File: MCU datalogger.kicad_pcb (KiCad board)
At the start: 2 copper layers, 50.8 x 30.5 mm, 29 parts, among them J1 Conn_01x04_Pin, J2 Conn_01x04_Pin, J3 Conn_01x09_Pin, J4 Conn_02x03_Odd_Even, U1 24LC1025, U2 24LC1025, U3 DS1337S_, U4 ATMEGA328P-AU, Y1 32.768 KHz, Y2 16 MHz

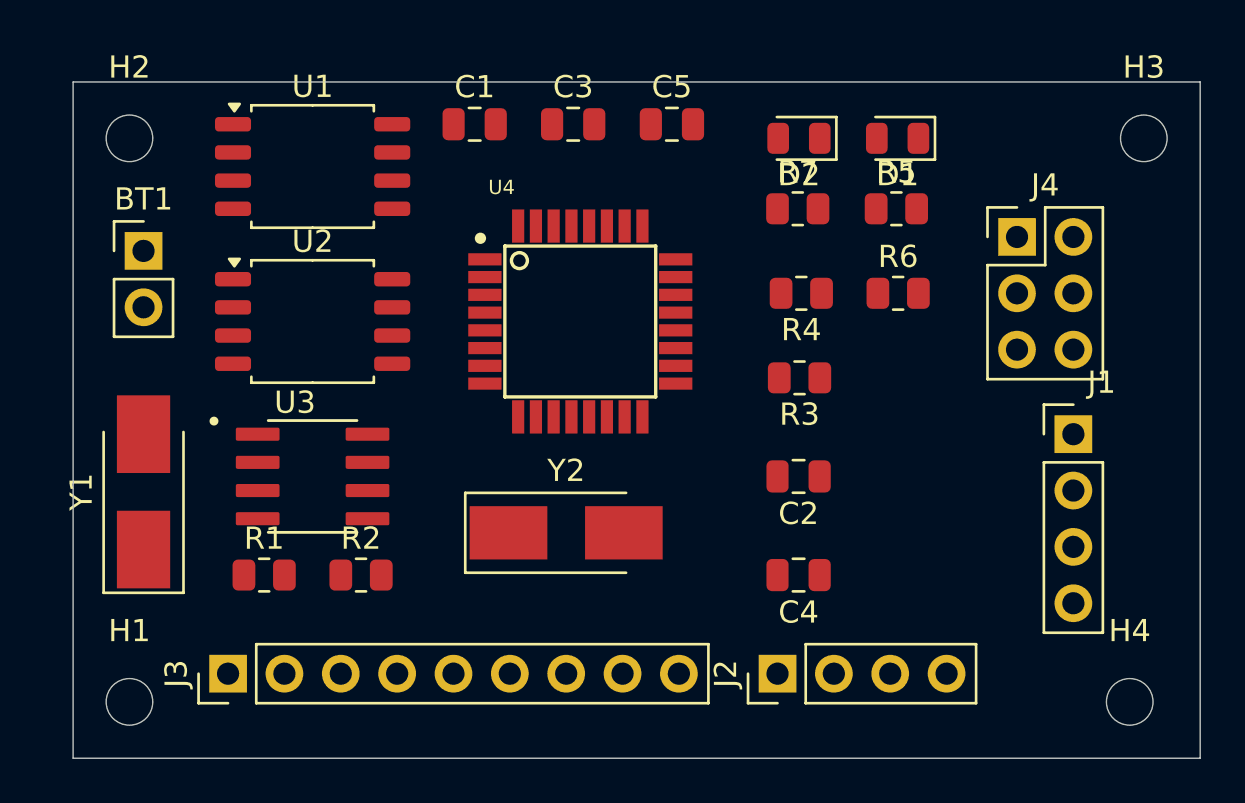
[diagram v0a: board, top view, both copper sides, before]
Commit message: Routing and GND Vcc complete
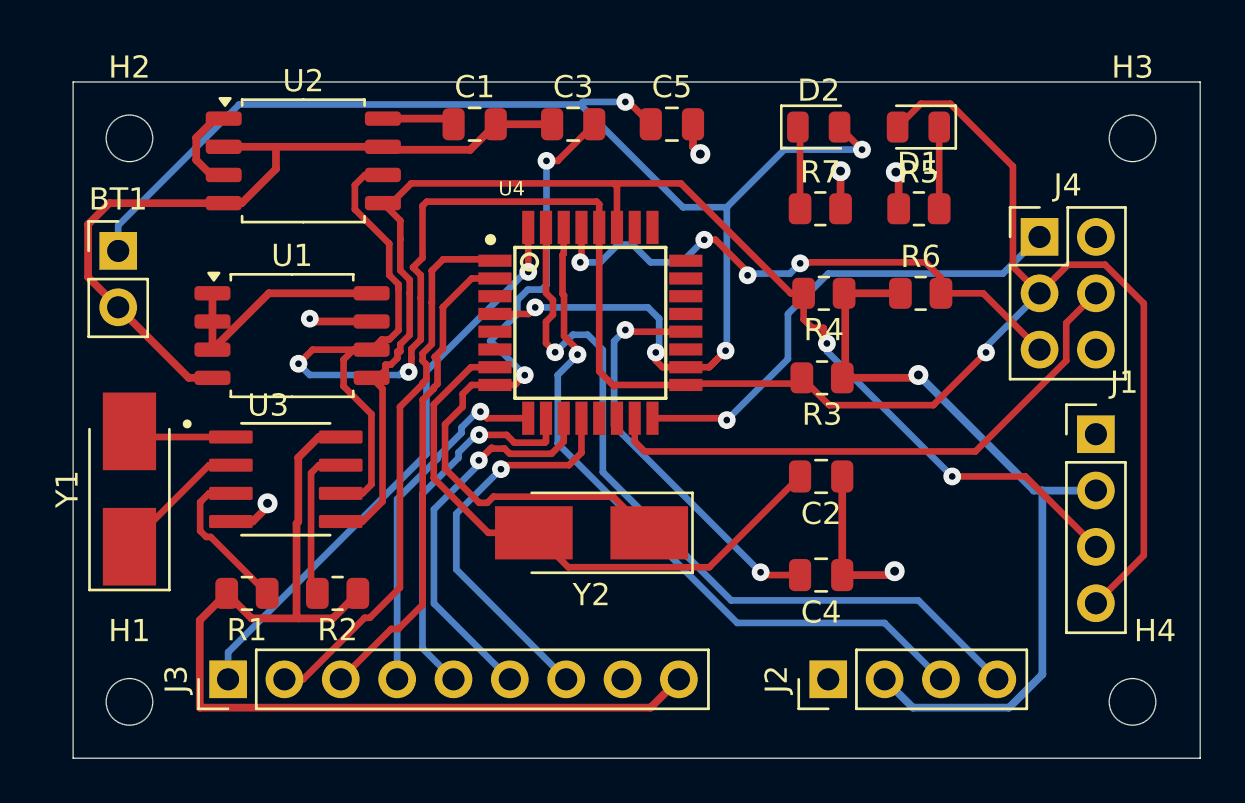
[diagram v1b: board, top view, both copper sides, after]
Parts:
- moved U1 7.68 mm to (73.4, 97.8)
- moved U2 7.25 mm to (73.9, 89.9)
- moved J2 2.30 mm to (97.5, 113.3)
- moved R2 1.34 mm to (75.4, 109.4), turned to 180 degrees
- moved U3 1.21 mm to (73.1, 104.3)
- moved BT1 1.14 mm to (65.5, 94.0)
- moved Y2 1.14 mm to (86.9, 106.7), turned to 180 degrees
- moved R1 1.13 mm to (71.3, 109.4), turned to 180 degrees
- moved D1 1.07 mm to (101.6, 88.4)
- moved D2 1.02 mm to (97.1, 88.4), turned to 0 degrees
- moved J1 1.02 mm to (109.6, 102.2)
- moved J4 1.02 mm to (107.1, 93.3)
- moved R5 1.02 mm to (101.6, 92.1)
- moved R6 1.02 mm to (101.7, 95.9)
- moved R7 1.02 mm to (97.2, 92.1)
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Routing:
- net /SCK: track 0.00 -> 108.8 mm, vias 0 -> 3
- net /Vcc: track 0.00 -> 99.8 mm, vias 0 -> 1
- net Net-(BT1-+): track 0.00 -> 65.9 mm, vias 0 -> 5
- net /SDA: track 0.00 -> 60.0 mm, vias 0 -> 2
- net GND: track 0.00 -> 52.5 mm, vias 0 -> 6
- net /TX: track 0.00 -> 36.0 mm, vias 0 -> 1
- net /RX: track 0.00 -> 32.1 mm, vias 0 -> 1
- net Net-(U4-PB7): track 0.00 -> 32.1 mm, vias 0 -> 2
- net Net-(U4-PB6): track 0.00 -> 26.6 mm
- net /RESET: track 0.00 -> 26.4 mm, vias 0 -> 4
- net /D2: track 0.00 -> 26.0 mm, vias 0 -> 1
- net /MOSI: track 0.00 -> 26.0 mm
- net /D3: track 0.00 -> 24.5 mm
- net /MISO: track 0.00 -> 22.1 mm, vias 0 -> 1
- net /D4: track 0.00 -> 21.9 mm
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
